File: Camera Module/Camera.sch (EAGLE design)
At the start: 8 parts, among them U2 RFM69HCW

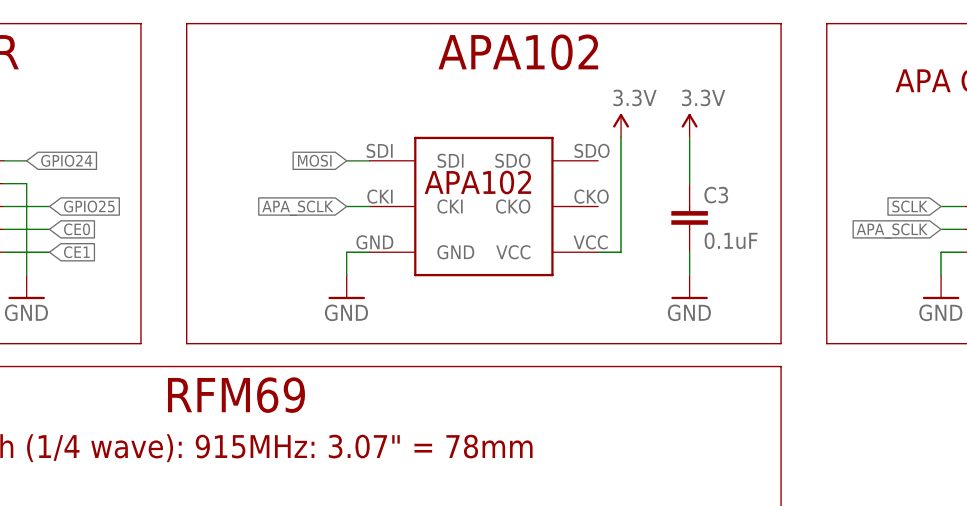
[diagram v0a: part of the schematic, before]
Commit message: Finalized all PCBs
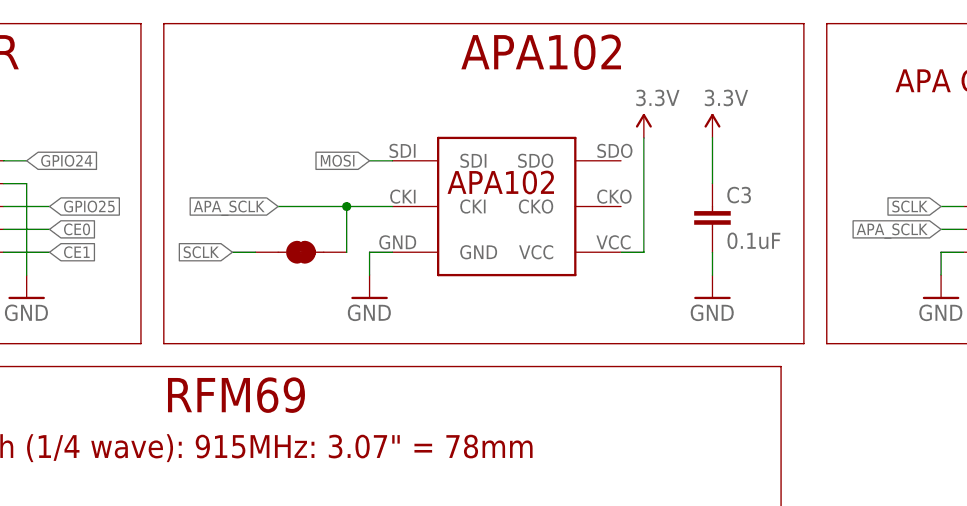
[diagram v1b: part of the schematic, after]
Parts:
- added JP1: JUMPER-PAD-2-NC_BY_TRACE, SparkFun-Passives:JUMPER-PAD-2-NC_BY_TRACE
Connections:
- net APA_SCLK: now also JP1.2
- net SCLK: now also JP1.1
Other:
- moved on the sheet: C3
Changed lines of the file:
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@@
 <part name="SUPPLY7" library="SparkFun-Aesthetics" deviceset="3.3V" device=""/>
 <part name="GND8" library="SparkFun-Aesthetics" deviceset="GND" device=""/>
+<part name="JP1" library="SparkFun-Passives" deviceset="JUMPER-PAD-2-NC_BY_TRACE" device=""/>
 </parts>
 <sheets>
@@
 <wire x1="43.18" y1="71.12" x2="0" y2="71.12" width="0.1524" layer="94"/>
 <wire x1="0" y1="71.12" x2="0" y2="106.68" width="0.1524" layer="94"/>
-<text x="76.2" y="101.6" size="3.81" layer="94">APA102</text>
-<wire x1="48.26" y1="106.68" x2="114.3" y2="106.68" width="0.1524" layer="94"/>
-<wire x1="114.3" y1="106.68" x2="114.3" y2="71.12" width="0.1524" layer="94"/>
-<wire x1="114.3" y1="71.12" x2="48.26" y2="71.12" width="0.1524" layer="94"/>
-<wire x1="48.26" y1="71.12" x2="48.26" y2="106.68" width="0.1524" layer="94"/>
+<text x="78.74" y="101.6" size="3.81" layer="94">APA102</text>
+<wire x1="45.72" y1="106.68" x2="116.84" y2="106.68" width="0.1524" layer="94"/>
+<wire x1="116.84" y1="106.68" x2="116.84" y2="71.12" width="0.1524" layer="94"/>
+<wire x1="116.84" y1="71.12" x2="45.72" y2="71.12" width="0.1524" layer="94"/>
+<wire x1="45.72" y1="71.12" x2="45.72" y2="106.68" width="0.1524" layer="94"/>
 <wire x1="119.38" y1="106.68" x2="119.38" y2="71.12" width="0.1524" layer="94"/>
 <wire x1="119.38" y1="71.12" x2="167.64" y2="71.12" width="0.1524" layer="94"/>
@@
 <instance part="GND4" gate="1" x="10.16" y="76.2"/>
 <instance part="GND5" gate="1" x="30.48" y="76.2"/>
-<instance part="U$1" gate="G$1" x="81.28" y="86.36"/>
-<instance part="GND6" gate="1" x="66.04" y="76.2"/>
-<instance part="SUPPLY5" gate="G$1" x="96.52" y="93.98"/>
-<instance part="C3" gate="G$1" x="104.14" y="83.82"/>
-<instance part="SUPPLY6" gate="G$1" x="104.14" y="93.98"/>
-<instance part="GND7" gate="1" x="104.14" y="76.2"/>
+<instance part="U$1" gate="G$1" x="83.82" y="86.36"/>
+<instance part="GND6" gate="1" x="68.58" y="76.2"/>
+<instance part="SUPPLY5" gate="G$1" x="99.06" y="93.98"/>
+<instance part="C3" gate="G$1" x="106.68" y="83.82"/>
+<instance part="SUPPLY6" gate="G$1" x="106.68" y="93.98"/>
+<instance part="GND7" gate="1" x="106.68" y="76.2"/>
 <instance part="U$2" gate="G$1" x="144.78" y="83.82"/>
 <instance part="SUPPLY7" gate="G$1" x="160.02" y="88.9"/>
 <instance part="GND8" gate="1" x="132.08" y="76.2"/>
+<instance part="JP1" gate="G$1" x="60.96" y="81.28" smashed="yes"/>
 </instances>
 <busses>
@@
 <segment>
 <pinref part="U$1" gate="G$1" pin="GND"/>
-<wire x1="68.58" y1="81.28" x2="66.04" y2="81.28" width="0.1524" layer="91"/>
+<wire x1="71.12" y1="81.28" x2="68.58" y2="81.28" width="0.1524" layer="91"/>
 <pinref part="GND6" gate="1" pin="GND"/>
-<wire x1="66.04" y1="81.28" x2="66.04" y2="78.74" width="0.1524" layer="91"/>
+<wire x1="68.58" y1="81.28" x2="68.58" y2="78.74" width="0.1524" layer="91"/>
 </segment>
 <segment>
 <pinref part="C3" gate="G$1" pin="2"/>
 <pinref part="GND7" gate="1" pin="GND"/>
-<wire x1="104.14" y1="78.74" x2="104.14" y2="81.28" width="0.1524" layer="91"/>
+<wire x1="106.68" y1="78.74" x2="106.68" y2="81.28" width="0.1524" layer="91"/>
 </segment>
 <segment>
@@
 <pinref part="U$1" gate="G$1" pin="VCC"/>
 <pinref part="SUPPLY5" gate="G$1" pin="3.3V"/>
-<wire x1="93.98" y1="81.28" x2="96.52" y2="81.28" width="0.1524" layer="91"/>
-<wire x1="96.52" y1="81.28" x2="96.52" y2="93.98" width="0.1524" layer="91"/>
+<wire x1="96.52" y1="81.28" x2="99.06" y2="81.28" width="0.1524" layer="91"/>
+<wire x1="99.06" y1="81.28" x2="99.06" y2="93.98" width="0.1524" layer="91"/>
 </segment>
 <segment>
 <pinref part="C3" gate="G$1" pin="1"/>
 <pinref part="SUPPLY6" gate="G$1" pin="3.3V"/>
-<wire x1="104.14" y1="93.98" x2="104.14" y2="88.9" width="0.1524" layer="91"/>
+<wire x1="106.68" y1="93.98" x2="106.68" y2="88.9" width="0.1524" layer="91"/>
 </segment>
 <segment>
@@
 <segment>
 <pinref part="U$1" gate="G$1" pin="SDI"/>
-<wire x1="68.58" y1="91.44" x2="66.04" y2="91.44" width="0.1524" layer="91"/>
-<label x="66.04" y="91.44" size="1.27" layer="95" rot="R180" xref="yes"/>
+<wire x1="71.12" y1="91.44" x2="68.58" y2="91.44" width="0.1524" layer="91"/>
+<label x="68.58" y="91.44" size="1.27" layer="95" rot="R180" xref="yes"/>
 </segment>
 <segment>
@@
 <label x="132.08" y="86.36" size="1.27" layer="95" rot="R180" xref="yes"/>
 </segment>
+<segment>
+<pinref part="JP1" gate="G$1" pin="1"/>
+<wire x1="55.88" y1="81.28" x2="53.34" y2="81.28" width="0.1524" layer="91"/>
+<label x="53.34" y="81.28" size="1.27" layer="95" rot="R180" xref="yes"/>
+</segment>
 </net>
 <net name="CE0" class="0">
@@
 <segment>
 <pinref part="U$1" gate="G$1" pin="CKI"/>
-<wire x1="68.58" y1="86.36" x2="66.04" y2="86.36" width="0.1524" layer="91"/>
-<label x="66.04" y="86.36" size="1.27" layer="95" rot="R180" xref="yes"/>
-</segment>
-<segment>
+<wire x1="71.12" y1="86.36" x2="66.04" y2="86.36" width="0.1524" layer="91"/>
+<label x="58.42" y="86.36" size="1.27" layer="95" rot="R180" xref="yes"/>
+<pinref part="JP1" gate="G$1" pin="2"/>
+<wire x1="66.04" y1="86.36" x2="58.42" y2="86.36" width="0.1524" layer="91"/>
+<wire x1="66.04" y1="86.36" x2="66.04" y2="81.28" width="0.1524" layer="91"/>
+<junction x="66.04" y="86.36"/>
+</segment>
+<segment>
